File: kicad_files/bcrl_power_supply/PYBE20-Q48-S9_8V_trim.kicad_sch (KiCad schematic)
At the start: 9 parts

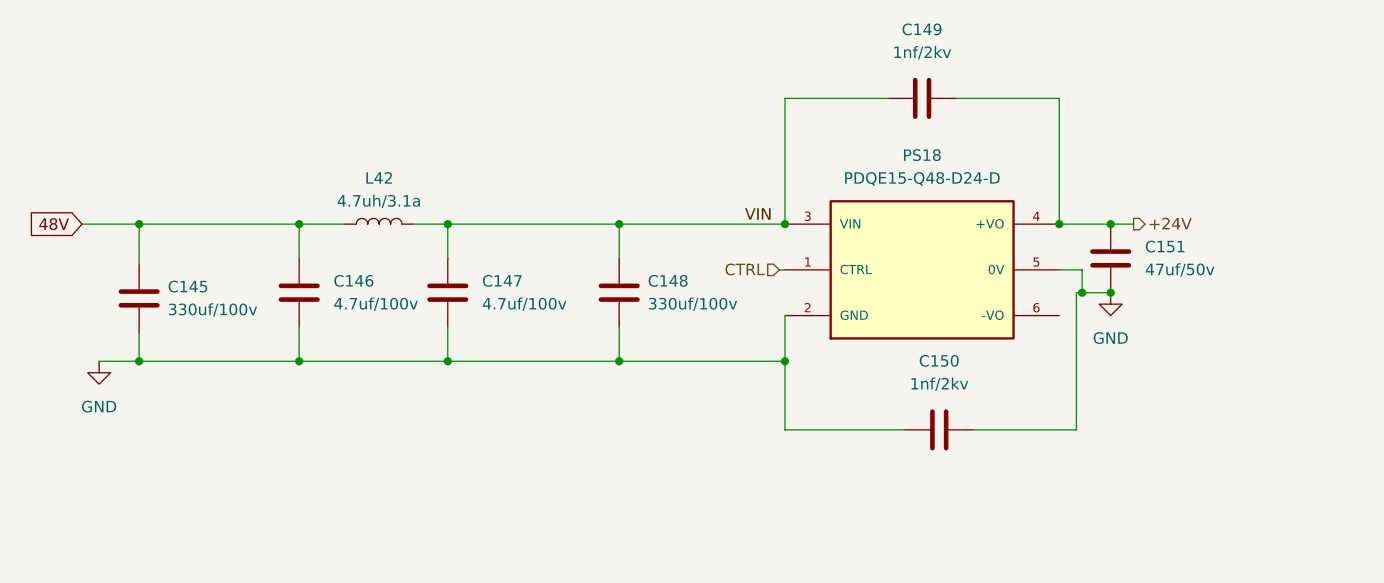
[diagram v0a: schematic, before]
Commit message: started LCSC, fixing DCDC
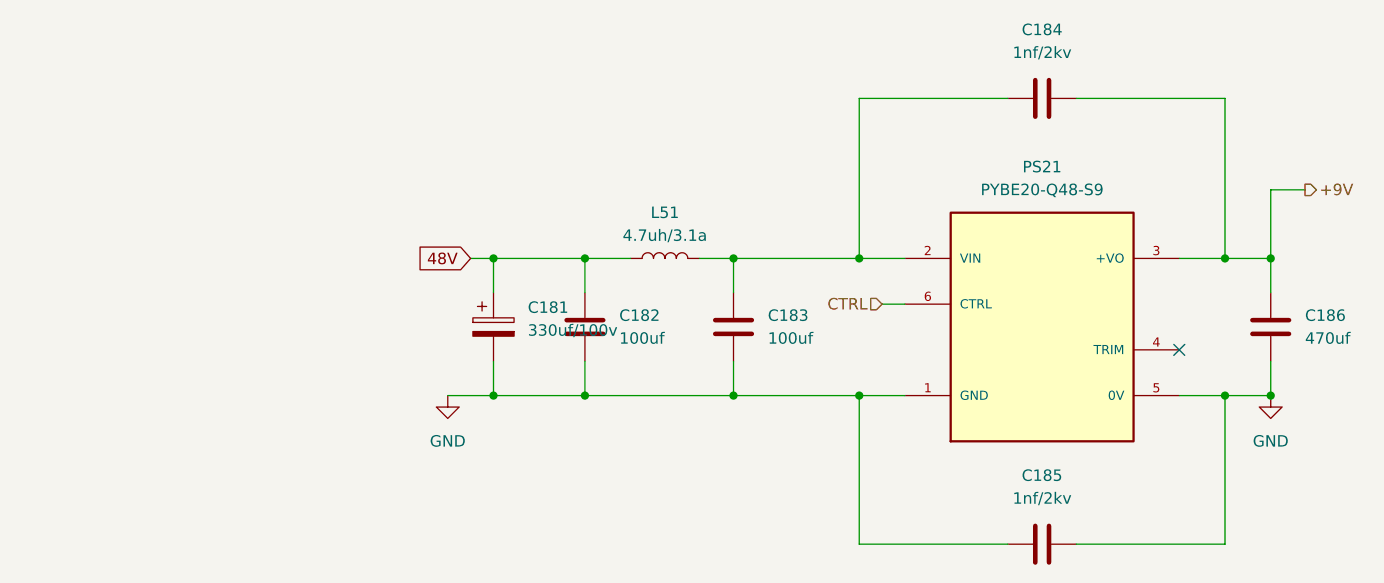
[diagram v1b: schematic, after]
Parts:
- removed C145, C148: 330uf/100v, Capacitor_SMD:C_0603_1608Metric, symbol Device:C
- removed C146, C147: 4.7uf/100v, Capacitor_SMD:C_0603_1608Metric, symbol Device:C
- removed C149, C150: 1nf/2kv, Capacitor_SMD:C_0603_1608Metric, symbol Device:C
- removed C151: 47uf/50v, Capacitor_SMD:C_0603_1608Metric, symbol Device:C
- removed L42: 4.7uh/3.1a, Inductor_SMD:L_0603_1608Metric, symbol Device:L
- removed PS18: PDQE15-Q48-D24-D, BCRL_power_supply:CONV_PDQE15-Q48-D24-D, symbol BCRL_power_supply:PDQE15-Q48-D24-D
- added C181: 330uf/100v, Capacitor_SMD:C_0603_1608Metric, symbol Device:C_Polarized
- added C182, C183: 100uf, Capacitor_SMD:C_0603_1608Metric, symbol Device:C
- added C184, C185: 1nf/2kv, Capacitor_SMD:C_0603_1608Metric, symbol Device:C
- added C186: 470uf, Capacitor_SMD:C_0603_1608Metric, symbol Device:C
- added L51: 4.7uh/3.1a, symbol Device:L
- added PS21: PYBE20-Q48-S9, symbol BCRL_power_supply:PYBE20-Q48-S9
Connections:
- net 48V: now also C181.1, C182.1, L51.1
- net CTRL: now also PS21.6 (CTRL)
- net GND: now also C181.2, C182.2, C183.2, C185.1, C185.2, C186.2, PS21.1 (GND), PS21.5 (0V)
- new net: C183.1, C184.1, L51.2, PS21.2 (VIN)
- new net +9V: C184.2, C186.1, PS21.3 (+VO)
- no-connect marks 0 -> 1
